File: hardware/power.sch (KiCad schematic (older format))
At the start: 12 parts, among them J2 V_MEAS, J3 A_MEAS, J4 5V_IN, J5 V_MEAS, J6 A_MEAS, J7 3V3_IN

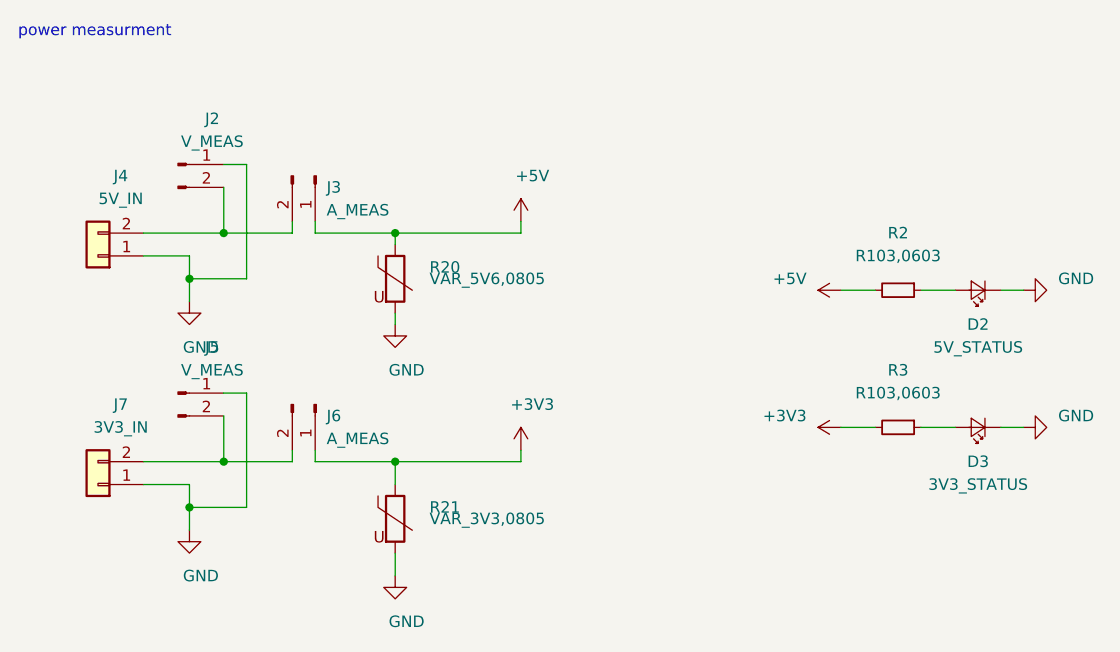
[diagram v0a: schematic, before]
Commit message: update,
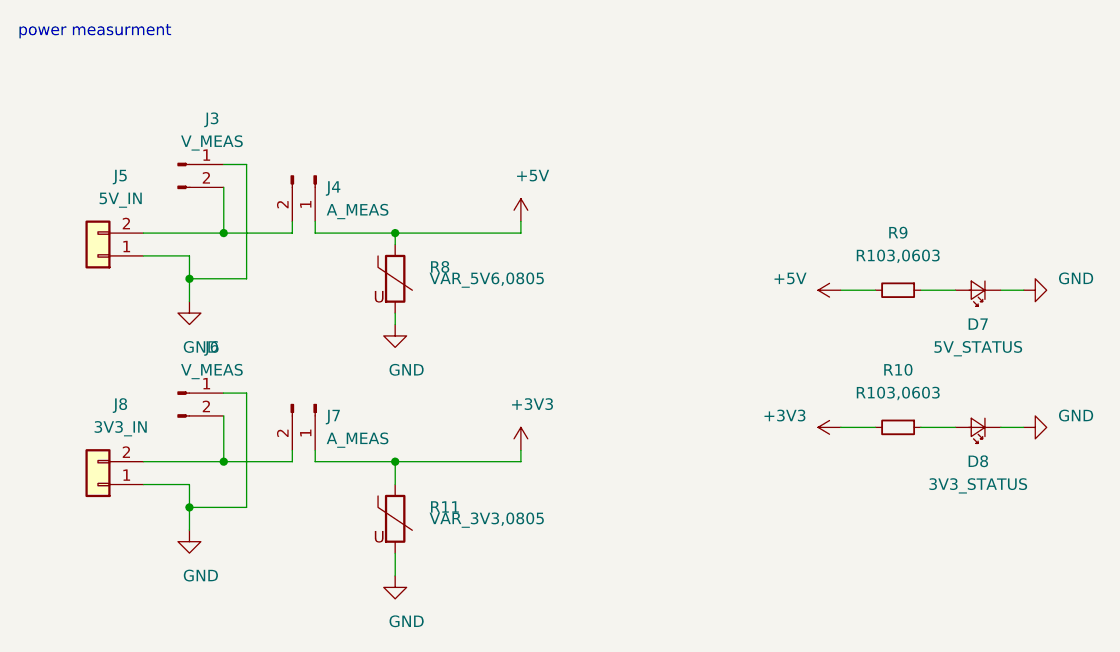
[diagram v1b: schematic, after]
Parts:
- renumbered D2 to D7, D3 to D8, J2 to J3, J3 to J4, J4 to J5, J5 to J6, J6 to J7, J7 to J8, R3 to R10, R21 to R11, R20 to R8, R2 to R9

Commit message: update,
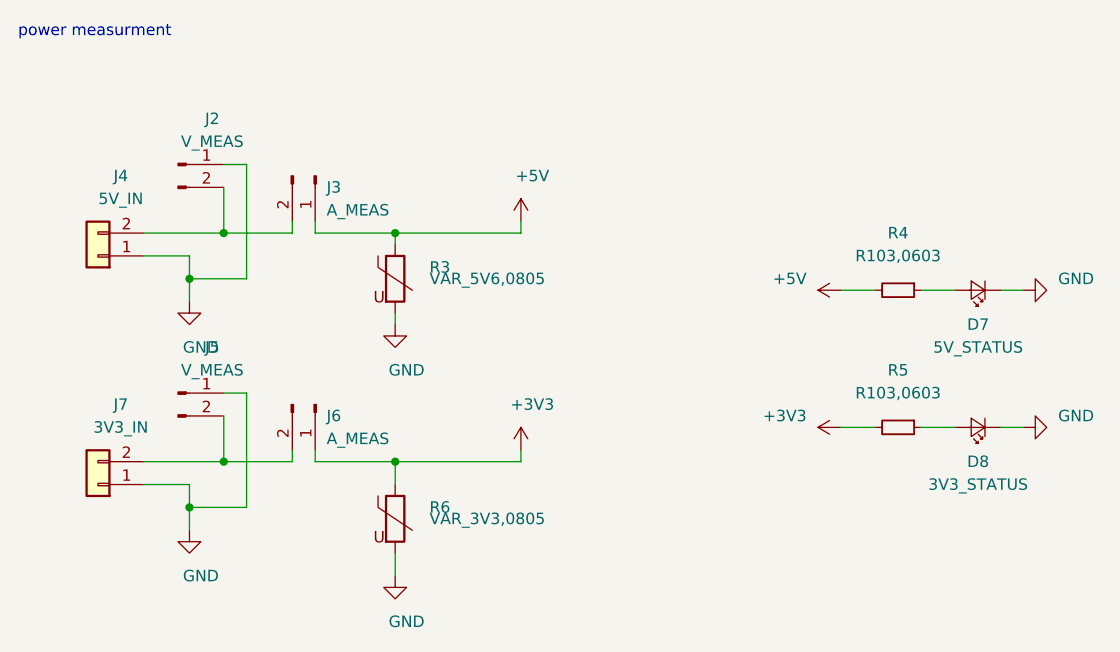
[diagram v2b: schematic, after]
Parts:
- renumbered J3 to J2, J4 to J3, J5 to J4, J6 to J5, J7 to J6, J8 to J7, R8 to R3, R9 to R4, R10 to R5, R11 to R6
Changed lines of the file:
@@
 $Descr User 8500 5500
 encoding utf-8
-Sheet 8 20
+Sheet 6 20
 Title ""
 Date ""
@@
 power measurment
 $Comp
-L Connector:Conn_01x02_Male J4
+L Connector:Conn_01x02_Male J3
 U 1 1 5CDC08AC
 P 2000 1450
-AR Path="/5CDAB997/5CDC08AC" Ref="J4"  Part="1"
+AR Path="/5CDAB997/5CDC08AC" Ref="J3"  Part="1"
 AR Path="/5CE8F13F/5CDC08AC" Ref="J?"  Part="1"
 AR Path="/5CDAB73D/5CF0E774/5CDC08AC" Ref="J?"  Part="1"
-F 0 "J4" V 2050 1500 50  0000 L CNN
+F 0 "J3" V 2050 1500 50  0000 L CNN
 F 1 "A_MEAS" V 2150 1500 50  0000 L CNN
 F 2 "" H 2000 1450 50  0001 C CNN
@@
 $EndComp
 $Comp
-L Connector_Generic:Conn_01x02 J5
+L Connector_Generic:Conn_01x02 J4
 U 1 1 5CDC1537
 P 1050 1800
-AR Path="/5CDAB997/5CDC1537" Ref="J5"  Part="1"
+AR Path="/5CDAB997/5CDC1537" Ref="J4"  Part="1"
 AR Path="/5CE8F13F/5CDC1537" Ref="J?"  Part="1"
 AR Path="/5CDAB73D/5CF0E774/5CDC1537" Ref="J?"  Part="1"
-F 0 "J5" H 950 1450 50  0000 C CNN
+F 0 "J4" H 950 1450 50  0000 C CNN
 F 1 "5V_IN" H 950 1550 50  0000 C CNN
 F 2 "" H 1050 1800 50  0001 C CNN
@@
 $EndComp
 $Comp
-L power:GND #PWR039
+L power:GND #PWR032
 U 1 1 5CDC1A75
 P 1450 2000
-AR Path="/5CDAB997/5CDC1A75" Ref="#PWR039"  Part="1"
+AR Path="/5CDAB997/5CDC1A75" Ref="#PWR032"  Part="1"
 AR Path="/5CE8F13F/5CDC1A75" Ref="#PWR?"  Part="1"
 AR Path="/5CDAB73D/5CF0E774/5CDC1A75" Ref="#PWR?"  Part="1"
-F 0 "#PWR039" H 1450 1750 50  0001 C CNN
+F 0 "#PWR032" H 1450 1750 50  0001 C CNN
 F 1 "GND" H 1500 1800 50  0000 C CNN
 F 2 "" H 1450 2000 50  0001 C CNN
@@
 	1450 1800 1450 1900
 $Comp
-L Connector:Conn_01x02_Male J3
+L Connector:Conn_01x02_Male J2
 U 1 1 5CDC22C8
 P 1400 1400
-AR Path="/5CDAB997/5CDC22C8" Ref="J3"  Part="1"
+AR Path="/5CDAB997/5CDC22C8" Ref="J2"  Part="1"
 AR Path="/5CE8F13F/5CDC22C8" Ref="J?"  Part="1"
 AR Path="/5CDAB73D/5CF0E774/5CDC22C8" Ref="J?"  Part="1"
-F 0 "J3" H 1550 1600 50  0000 C CNN
+F 0 "J2" H 1550 1600 50  0000 C CNN
 F 1 "V_MEAS" H 1550 1500 50  0000 C CNN
 F 2 "" H 1400 1400 50  0001 C CNN
@@
 Connection ~ 1600 1700
 $Comp
-L power:+5V #PWR036
+L power:+5V #PWR029
 U 1 1 5CDC5556
 P 2900 1650
-AR Path="/5CDAB997/5CDC5556" Ref="#PWR036"  Part="1"
+AR Path="/5CDAB997/5CDC5556" Ref="#PWR029"  Part="1"
 AR Path="/5CE8F13F/5CDC5556" Ref="#PWR?"  Part="1"
 AR Path="/5CDAB73D/5CF0E774/5CDC5556" Ref="#PWR?"  Part="1"
-F 0 "#PWR036" H 2900 1500 50  0001 C CNN
+F 0 "#PWR029" H 2900 1500 50  0001 C CNN
 F 1 "+5V" H 2950 1850 50  0000 C CNN
 F 2 "" H 2900 1650 50  0001 C CNN
@@
 	2000 1700 2000 1650
 $Comp
-L Connector:Conn_01x02_Male J7
+L Connector:Conn_01x02_Male J6
 U 1 1 5CDC6A22
 P 2000 2450
-AR Path="/5CDAB997/5CDC6A22" Ref="J7"  Part="1"
+AR Path="/5CDAB997/5CDC6A22" Ref="J6"  Part="1"
 AR Path="/5CE8F13F/5CDC6A22" Ref="J?"  Part="1"
 AR Path="/5CDAB73D/5CF0E774/5CDC6A22" Ref="J?"  Part="1"
-F 0 "J7" V 2050 2500 50  0000 L CNN
+F 0 "J6" V 2050 2500 50  0000 L CNN
 F 1 "A_MEAS" V 2150 2500 50  0000 L CNN
 F 2 "" H 2000 2450 50  0001 C CNN
@@
 $EndComp
 $Comp
-L Connector_Generic:Conn_01x02 J8
+L Connector_Generic:Conn_01x02 J7
 U 1 1 5CDC6A2C
 P 1050 2800
-AR Path="/5CDAB997/5CDC6A2C" Ref="J8"  Part="1"
+AR Path="/5CDAB997/5CDC6A2C" Ref="J7"  Part="1"
 AR Path="/5CE8F13F/5CDC6A2C" Ref="J?"  Part="1"
 AR Path="/5CDAB73D/5CF0E774/5CDC6A2C" Ref="J?"  Part="1"
-F 0 "J8" H 950 2450 50  0000 C CNN
+F 0 "J7" H 950 2450 50  0000 C CNN
 F 1 "3V3_IN" H 950 2550 50  0000 C CNN
 F 2 "" H 1050 2800 50  0001 C CNN
@@
 $EndComp
 $Comp
-L power:GND #PWR044
+L power:GND #PWR037
 U 1 1 5CDC6A36
 P 1450 3000
-AR Path="/5CDAB997/5CDC6A36" Ref="#PWR044"  Part="1"
+AR Path="/5CDAB997/5CDC6A36" Ref="#PWR037"  Part="1"
 AR Path="/5CE8F13F/5CDC6A36" Ref="#PWR?"  Part="1"
 AR Path="/5CDAB73D/5CF0E774/5CDC6A36" Ref="#PWR?"  Part="1"
-F 0 "#PWR044" H 1450 2750 50  0001 C CNN
+F 0 "#PWR037" H 1450 2750 50  0001 C CNN
 F 1 "GND" H 1500 2800 50  0000 C CNN
 F 2 "" H 1450 3000 50  0001 C CNN
@@
 	1450 2800 1450 2900
 $Comp
-L Connector:Conn_01x02_Male J6
+L Connector:Conn_01x02_Male J5
 U 1 1 5CDC6A42
 P 1400 2400
-AR Path="/5CDAB997/5CDC6A42" Ref="J6"  Part="1"
+AR Path="/5CDAB997/5CDC6A42" Ref="J5"  Part="1"
 AR Path="/5CE8F13F/5CDC6A42" Ref="J?"  Part="1"
 AR Path="/5CDAB73D/5CF0E774/5CDC6A42" Ref="J?"  Part="1"
-F 0 "J6" H 1550 2600 50  0000 C CNN
+F 0 "J5" H 1550 2600 50  0000 C CNN
 F 1 "V_MEAS" H 1550 2500 50  0000 C CNN
 F 2 "" H 1400 2400 50  0001 C CNN
@@
 	2000 2700 2000 2650
 $Comp
-L power:+3V3 #PWR043
+L power:+3V3 #PWR036
 U 1 1 5CDC8B9F
 P 2900 2650
-AR Path="/5CDAB997/5CDC8B9F" Ref="#PWR043"  Part="1"
+AR Path="/5CDAB997/5CDC8B9F" Ref="#PWR036"  Part="1"
 AR Path="/5CE8F13F/5CDC8B9F" Ref="#PWR?"  Part="1"
 AR Path="/5CDAB73D/5CF0E774/5CDC8B9F" Ref="#PWR?"  Part="1"
-F 0 "#PWR043" H 2900 2500 50  0001 C CNN
+F 0 "#PWR036" H 2900 2500 50  0001 C CNN
 F 1 "+3V3" H 2950 2850 50  0000 C CNN
 F 2 "" H 2900 2650 50  0001 C CNN
@@
 $EndComp
 $Comp
-L power:+5V #PWR037
+L power:+5V #PWR030
 U 1 1 5CDD6EE1
 P 4300 1950
-AR Path="/5CDAB997/5CDD6EE1" Ref="#PWR037"  Part="1"
+AR Path="/5CDAB997/5CDD6EE1" Ref="#PWR030"  Part="1"
 AR Path="/5CE8F13F/5CDD6EE1" Ref="#PWR?"  Part="1"
 AR Path="/5CDAB73D/5CF0E774/5CDD6EE1" Ref="#PWR?"  Part="1"
-F 0 "#PWR037" H 4300 1800 50  0001 C CNN
+F 0 "#PWR030" H 4300 1800 50  0001 C CNN
 F 1 "+5V" V 4350 2100 50  0000 L CNN
 F 2 "" H 4300 1950 50  0001 C CNN
@@
 $EndComp
 $Comp
-L taobao-r:R103,0603 R9
+L taobao-r:R103,0603 R4
 U 1 1 5CDD7398
 P 4550 1950
-AR Path="/5CDAB997/5CDD7398" Ref="R9"  Part="1"
+AR Path="/5CDAB997/5CDD7398" Ref="R4"  Part="1"
 AR Path="/5CE8F13F/5CDD7398" Ref="R?"  Part="1"
 AR Path="/5CDAB73D/5CF0E774/5CDD7398" Ref="R?"  Part="1"
-F 0 "R9" V 4300 1950 50  0000 C CNN
+F 0 "R4" V 4300 1950 50  0000 C CNN
 F 1 "R103,0603" V 4400 1950 50  0000 C CNN
 F 2 "Resistor_SMD:R_0603_1608Metric_Pad1.05x0.95mm_HandSolder" H 4550 1950 50  0001 C CNN
@@
 $EndComp
 $Comp
-L power:GND #PWR038
+L power:GND #PWR031
 U 1 1 5CDD83E9
 P 5100 1950
-AR Path="/5CDAB997/5CDD83E9" Ref="#PWR038"  Part="1"
+AR Path="/5CDAB997/5CDD83E9" Ref="#PWR031"  Part="1"
 AR Path="/5CE8F13F/5CDD83E9" Ref="#PWR?"  Part="1"
 AR Path="/5CDAB73D/5CF0E774/5CDD83E9" Ref="#PWR?"  Part="1"
-F 0 "#PWR038" H 5100 1700 50  0001 C CNN
+F 0 "#PWR031" H 5100 1700 50  0001 C CNN
 F 1 "GND" V 5150 1800 50  0000 R CNN
 F 2 "" H 5100 1950 50  0001 C CNN
@@
 	5000 1950 5100 1950
 $Comp
-L taobao-r:R103,0603 R10
+L taobao-r:R103,0603 R5
 U 1 1 5CDDC8A9
 P 4550 2550
-AR Path="/5CDAB997/5CDDC8A9" Ref="R10"  Part="1"
+AR Path="/5CDAB997/5CDDC8A9" Ref="R5"  Part="1"
 AR Path="/5CE8F13F/5CDDC8A9" Ref="R?"  Part="1"
 AR Path="/5CDAB73D/5CF0E774/5CDDC8A9" Ref="R?"  Part="1"
-F 0 "R10" V 4300 2550 50  0000 C CNN
+F 0 "R5" V 4300 2550 50  0000 C CNN
 F 1 "R103,0603" V 4400 2550 50  0000 C CNN
 F 2 "Resistor_SMD:R_0603_1608Metric_Pad1.05x0.95mm_HandSolder" H 4550 2550 50  0001 C CNN
@@
 $EndComp
 $Comp
-L power:GND #PWR042
+L power:GND #PWR035
 U 1 1 5CDDC8BD
 P 5100 2550
-AR Path="/5CDAB997/5CDDC8BD" Ref="#PWR042"  Part="1"
+AR Path="/5CDAB997/5CDDC8BD" Ref="#PWR035"  Part="1"
 AR Path="/5CE8F13F/5CDDC8BD" Ref="#PWR?"  Part="1"
 AR Path="/5CDAB73D/5CF0E774/5CDDC8BD" Ref="#PWR?"  Part="1"
-F 0 "#PWR042" H 5100 2300 50  0001 C CNN
+F 0 "#PWR035" H 5100 2300 50  0001 C CNN
 F 1 "GND" V 5150 2400 50  0000 R CNN
 F 2 "" H 5100 2550 50  0001 C CNN
@@
 	5000 2550 5100 2550
 $Comp
-L power:+3V3 #PWR041
+L power:+3V3 #PWR034
 U 1 1 5CDDDD9C
 P 4300 2550
-AR Path="/5CDAB997/5CDDDD9C" Ref="#PWR041"  Part="1"
+AR Path="/5CDAB997/5CDDDD9C" Ref="#PWR034"  Part="1"
 AR Path="/5CE8F13F/5CDDDD9C" Ref="#PWR?"  Part="1"
 AR Path="/5CDAB73D/5CF0E774/5CDDDD9C" Ref="#PWR?"  Part="1"
-F 0 "#PWR041" H 4300 2400 50  0001 C CNN
+F 0 "#PWR034" H 4300 2400 50  0001 C CNN
 F 1 "+3V3" V 4350 2700 50  0000 L CNN
 F 2 "" H 4300 2550 50  0001 C CNN
@@
 $EndComp
 $Comp
-L taobao-varistor:VAR_5V6,0805 R8
+L taobao-varistor:VAR_5V6,0805 R3
 U 1 1 5CE50EF8
 P 2350 1900
-AR Path="/5CDAB997/5CE50EF8" Ref="R8"  Part="1"
+AR Path="/5CDAB997/5CE50EF8" Ref="R3"  Part="1"
 AR Path="/5CDAB73D/5CF0E774/5CE50EF8" Ref="R?"  Part="1"
-F 0 "R8" H 2500 1950 50  0000 L CNN
+F 0 "R3" H 2500 1950 50  0000 L CNN
 F 1 "VAR_5V6,0805" H 2500 1900 50  0000 L CNN
 F 2 "footprint-lib:VAR_0805" H 2350 1900 50  0001 C CNN
@@
 	2350 1700 2000 1700
 $Comp
-L power:GND #PWR040
+L power:GND #PWR033
 U 1 1 5CE517F1
 P 2350 2100
-AR Path="/5CDAB997/5CE517F1" Ref="#PWR040"  Part="1"
+AR Path="/5CDAB997/5CE517F1" Ref="#PWR033"  Part="1"
 AR Path="/5CE8F13F/5CE517F1" Ref="#PWR?"  Part="1"
 AR Path="/5CDAB73D/5CF0E774/5CE517F1" Ref="#PWR?"  Part="1"
-F 0 "#PWR040" H 2350 1850 50  0001 C CNN
+F 0 "#PWR033" H 2350 1850 50  0001 C CNN
 F 1 "GND" H 2400 1900 50  0000 C CNN
 F 2 "" H 2350 2100 50  0001 C CNN
@@
 	2350 2050 2350 2100
 $Comp
-L taobao-varistor:VAR_3V3,0805 R11
+L taobao-varistor:VAR_3V3,0805 R6
 U 1 1 5CE538D7
 P 2350 2950
-AR Path="/5CDAB997/5CE538D7" Ref="R11"  Part="1"
+AR Path="/5CDAB997/5CE538D7" Ref="R6"  Part="1"
 AR Path="/5CDAB73D/5CF0E774/5CE538D7" Ref="R?"  Part="1"
-F 0 "R11" H 2500 3000 50  0000 L CNN
+F 0 "R6" H 2500 3000 50  0000 L CNN
 F 1 "VAR_3V3,0805" H 2500 2950 50  0000 L CNN
 F 2 "footprint-lib:VAR_0805" H 2350 2950 50  0001 C CNN
@@
 	2350 2700 2000 2700
 $Comp
-L power:GND #PWR045
+L power:GND #PWR038
 U 1 1 5CE5450B
 P 2350 3200
-AR Path="/5CDAB997/5CE5450B" Ref="#PWR045"  Part="1"
+AR Path="/5CDAB997/5CE5450B" Ref="#PWR038"  Part="1"
 AR Path="/5CDAB73D/5CF0E774/5CE5450B" Ref="#PWR?"  Part="1"
-F 0 "#PWR045" H 2350 2950 50  0001 C CNN
+F 0 "#PWR038" H 2350 2950 50  0001 C CNN
 F 1 "GND" H 2400 3000 50  0000 C CNN
 F 2 "" H 2350 3200 50  0001 C CNN

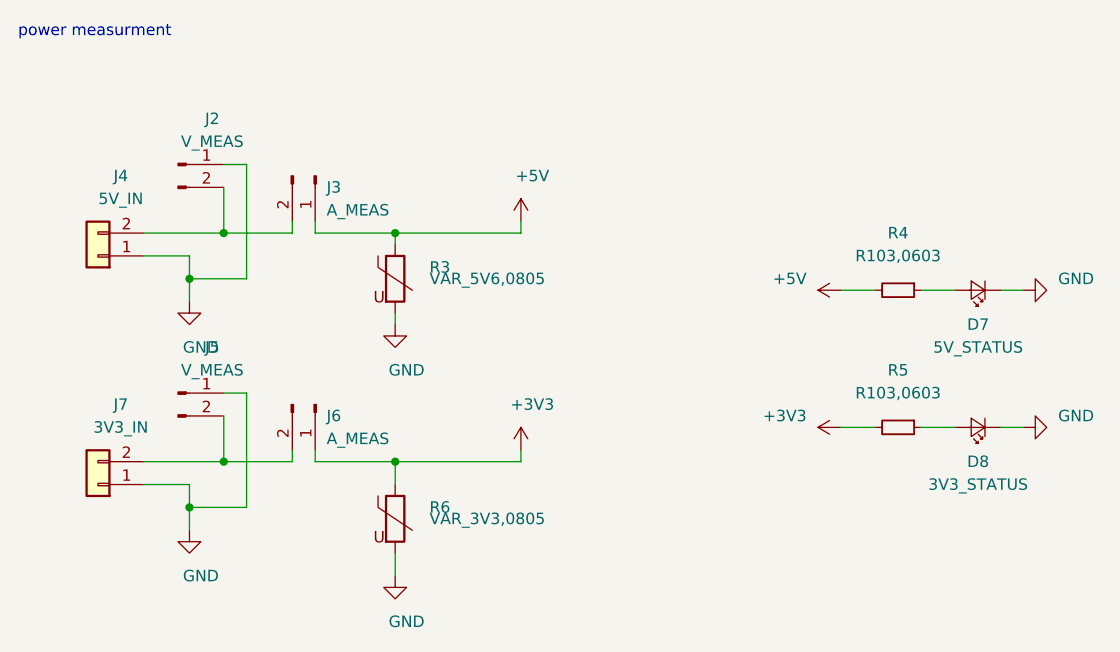
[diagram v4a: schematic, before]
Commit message: update,
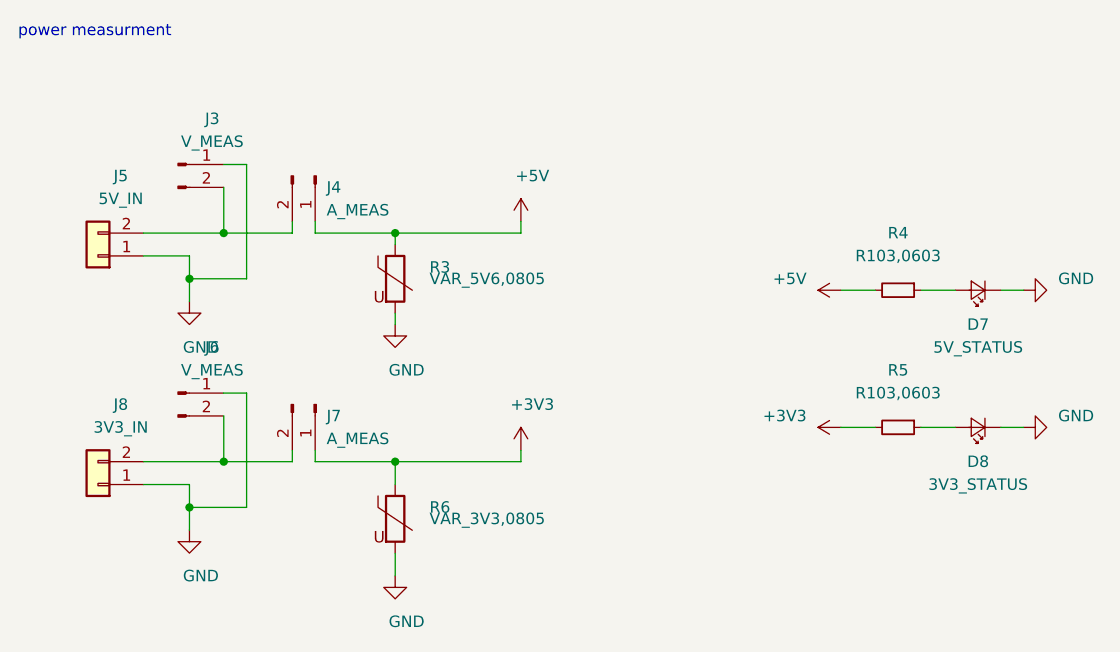
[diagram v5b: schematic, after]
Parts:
- renumbered J2 to J3, J3 to J4, J4 to J5, J5 to J6, J6 to J7, J7 to J8
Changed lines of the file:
@@
 power measurment
 $Comp
-L Connector:Conn_01x02_Male J3
+L Connector:Conn_01x02_Male J4
 U 1 1 5CDC08AC
 P 2000 1450
-AR Path="/5CDAB997/5CDC08AC" Ref="J3"  Part="1"
+AR Path="/5CDAB997/5CDC08AC" Ref="J4"  Part="1"
 AR Path="/5CE8F13F/5CDC08AC" Ref="J?"  Part="1"
 AR Path="/5CDAB73D/5CF0E774/5CDC08AC" Ref="J?"  Part="1"
-F 0 "J3" V 2050 1500 50  0000 L CNN
+F 0 "J4" V 2050 1500 50  0000 L CNN
 F 1 "A_MEAS" V 2150 1500 50  0000 L CNN
 F 2 "" H 2000 1450 50  0001 C CNN
@@
 $EndComp
 $Comp
-L Connector_Generic:Conn_01x02 J4
+L Connector_Generic:Conn_01x02 J5
 U 1 1 5CDC1537
 P 1050 1800
-AR Path="/5CDAB997/5CDC1537" Ref="J4"  Part="1"
+AR Path="/5CDAB997/5CDC1537" Ref="J5"  Part="1"
 AR Path="/5CE8F13F/5CDC1537" Ref="J?"  Part="1"
 AR Path="/5CDAB73D/5CF0E774/5CDC1537" Ref="J?"  Part="1"
-F 0 "J4" H 950 1450 50  0000 C CNN
+F 0 "J5" H 950 1450 50  0000 C CNN
 F 1 "5V_IN" H 950 1550 50  0000 C CNN
 F 2 "" H 1050 1800 50  0001 C CNN
@@
 	1450 1800 1450 1900
 $Comp
-L Connector:Conn_01x02_Male J2
+L Connector:Conn_01x02_Male J3
 U 1 1 5CDC22C8
 P 1400 1400
-AR Path="/5CDAB997/5CDC22C8" Ref="J2"  Part="1"
+AR Path="/5CDAB997/5CDC22C8" Ref="J3"  Part="1"
 AR Path="/5CE8F13F/5CDC22C8" Ref="J?"  Part="1"
 AR Path="/5CDAB73D/5CF0E774/5CDC22C8" Ref="J?"  Part="1"
-F 0 "J2" H 1550 1600 50  0000 C CNN
+F 0 "J3" H 1550 1600 50  0000 C CNN
 F 1 "V_MEAS" H 1550 1500 50  0000 C CNN
 F 2 "" H 1400 1400 50  0001 C CNN
@@
 	2000 1700 2000 1650
 $Comp
-L Connector:Conn_01x02_Male J6
+L Connector:Conn_01x02_Male J7
 U 1 1 5CDC6A22
 P 2000 2450
-AR Path="/5CDAB997/5CDC6A22" Ref="J6"  Part="1"
+AR Path="/5CDAB997/5CDC6A22" Ref="J7"  Part="1"
 AR Path="/5CE8F13F/5CDC6A22" Ref="J?"  Part="1"
 AR Path="/5CDAB73D/5CF0E774/5CDC6A22" Ref="J?"  Part="1"
-F 0 "J6" V 2050 2500 50  0000 L CNN
+F 0 "J7" V 2050 2500 50  0000 L CNN
 F 1 "A_MEAS" V 2150 2500 50  0000 L CNN
 F 2 "" H 2000 2450 50  0001 C CNN
@@
 $EndComp
 $Comp
-L Connector_Generic:Conn_01x02 J7
+L Connector_Generic:Conn_01x02 J8
 U 1 1 5CDC6A2C
 P 1050 2800
-AR Path="/5CDAB997/5CDC6A2C" Ref="J7"  Part="1"
+AR Path="/5CDAB997/5CDC6A2C" Ref="J8"  Part="1"
 AR Path="/5CE8F13F/5CDC6A2C" Ref="J?"  Part="1"
 AR Path="/5CDAB73D/5CF0E774/5CDC6A2C" Ref="J?"  Part="1"
-F 0 "J7" H 950 2450 50  0000 C CNN
+F 0 "J8" H 950 2450 50  0000 C CNN
 F 1 "3V3_IN" H 950 2550 50  0000 C CNN
 F 2 "" H 1050 2800 50  0001 C CNN
@@
 	1450 2800 1450 2900
 $Comp
-L Connector:Conn_01x02_Male J5
+L Connector:Conn_01x02_Male J6
 U 1 1 5CDC6A42
 P 1400 2400
-AR Path="/5CDAB997/5CDC6A42" Ref="J5"  Part="1"
+AR Path="/5CDAB997/5CDC6A42" Ref="J6"  Part="1"
 AR Path="/5CE8F13F/5CDC6A42" Ref="J?"  Part="1"
 AR Path="/5CDAB73D/5CF0E774/5CDC6A42" Ref="J?"  Part="1"
-F 0 "J5" H 1550 2600 50  0000 C CNN
+F 0 "J6" H 1550 2600 50  0000 C CNN
 F 1 "V_MEAS" H 1550 2500 50  0000 C CNN
 F 2 "" H 1400 2400 50  0001 C CNN
